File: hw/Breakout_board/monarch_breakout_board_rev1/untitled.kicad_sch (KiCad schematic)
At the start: 10 parts, among them J1 5037630491, J2 5037630291, J3 5037630291, J4 5037630291, J5 5037630291, J6 5037630291

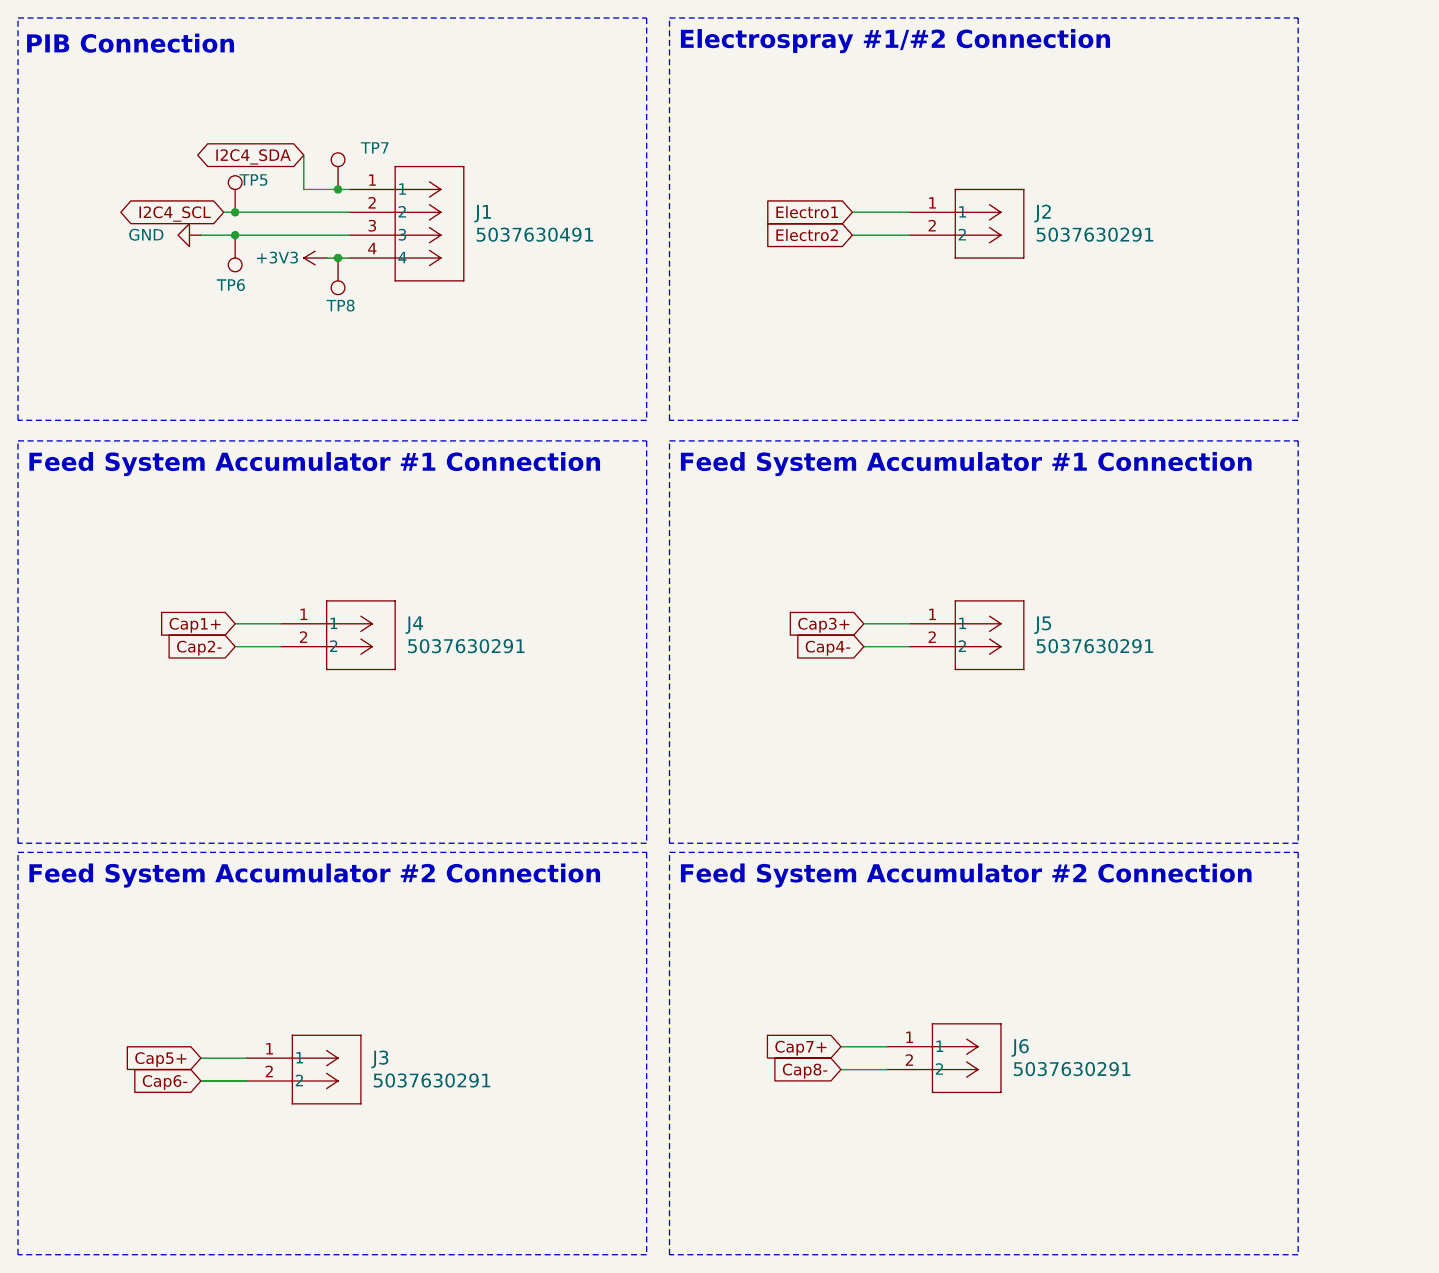
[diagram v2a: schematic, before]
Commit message: Final Breakout Board Work
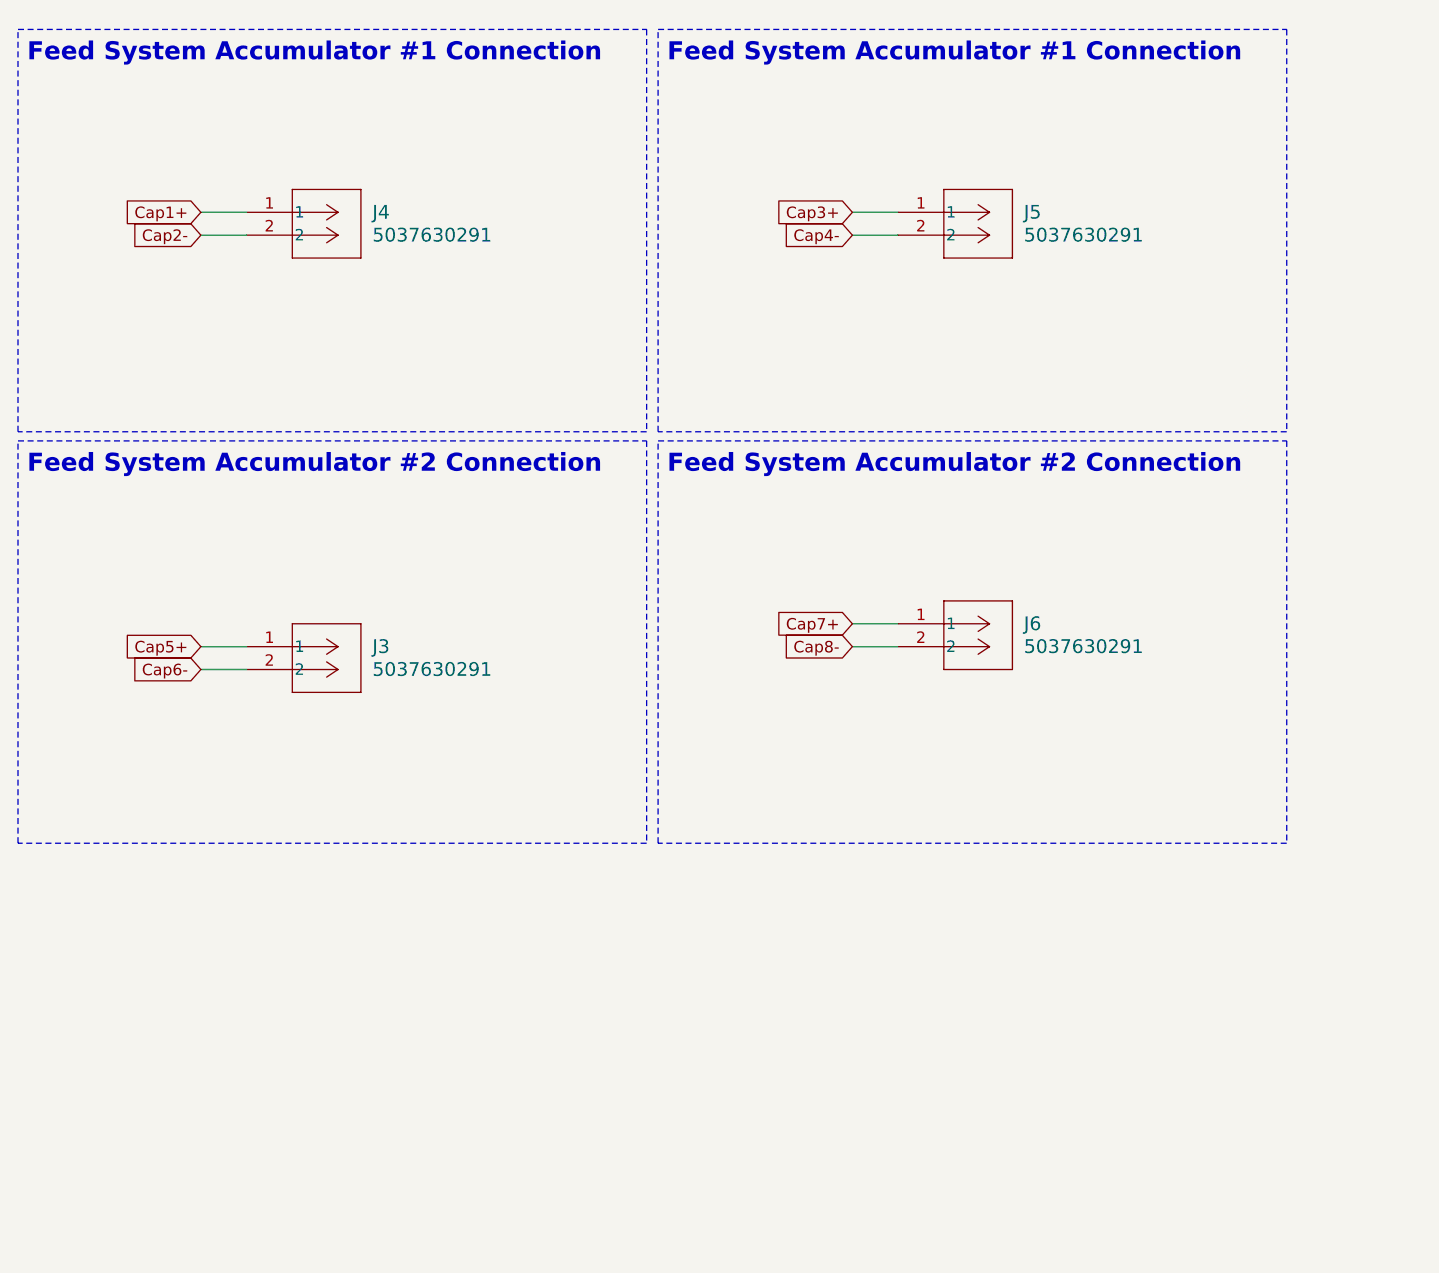
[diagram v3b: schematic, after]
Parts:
- removed J1: 5037630491, Connector 4 Pin:CONN_5037630000-SD_04_MOL, symbol 5037630491:5037630491
- removed J2: 5037630291, Connector 2 Pin:CONN_5037630000-SD_02_MOL, symbol Connectors 2 Pin:5037630291
- removed TP5, TP6, TP7, TP8: TestPoint, TestPoint:TestPoint_2Pads_Pitch2.54mm_Drill0.8mm, symbol Connector:TestPoint
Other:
- note removed: "Electrospray #1/#2 Connection"
- note removed: "PIB Connection"
- moved on the sheet: J3, J4, J5, J6

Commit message: FIXES after Review
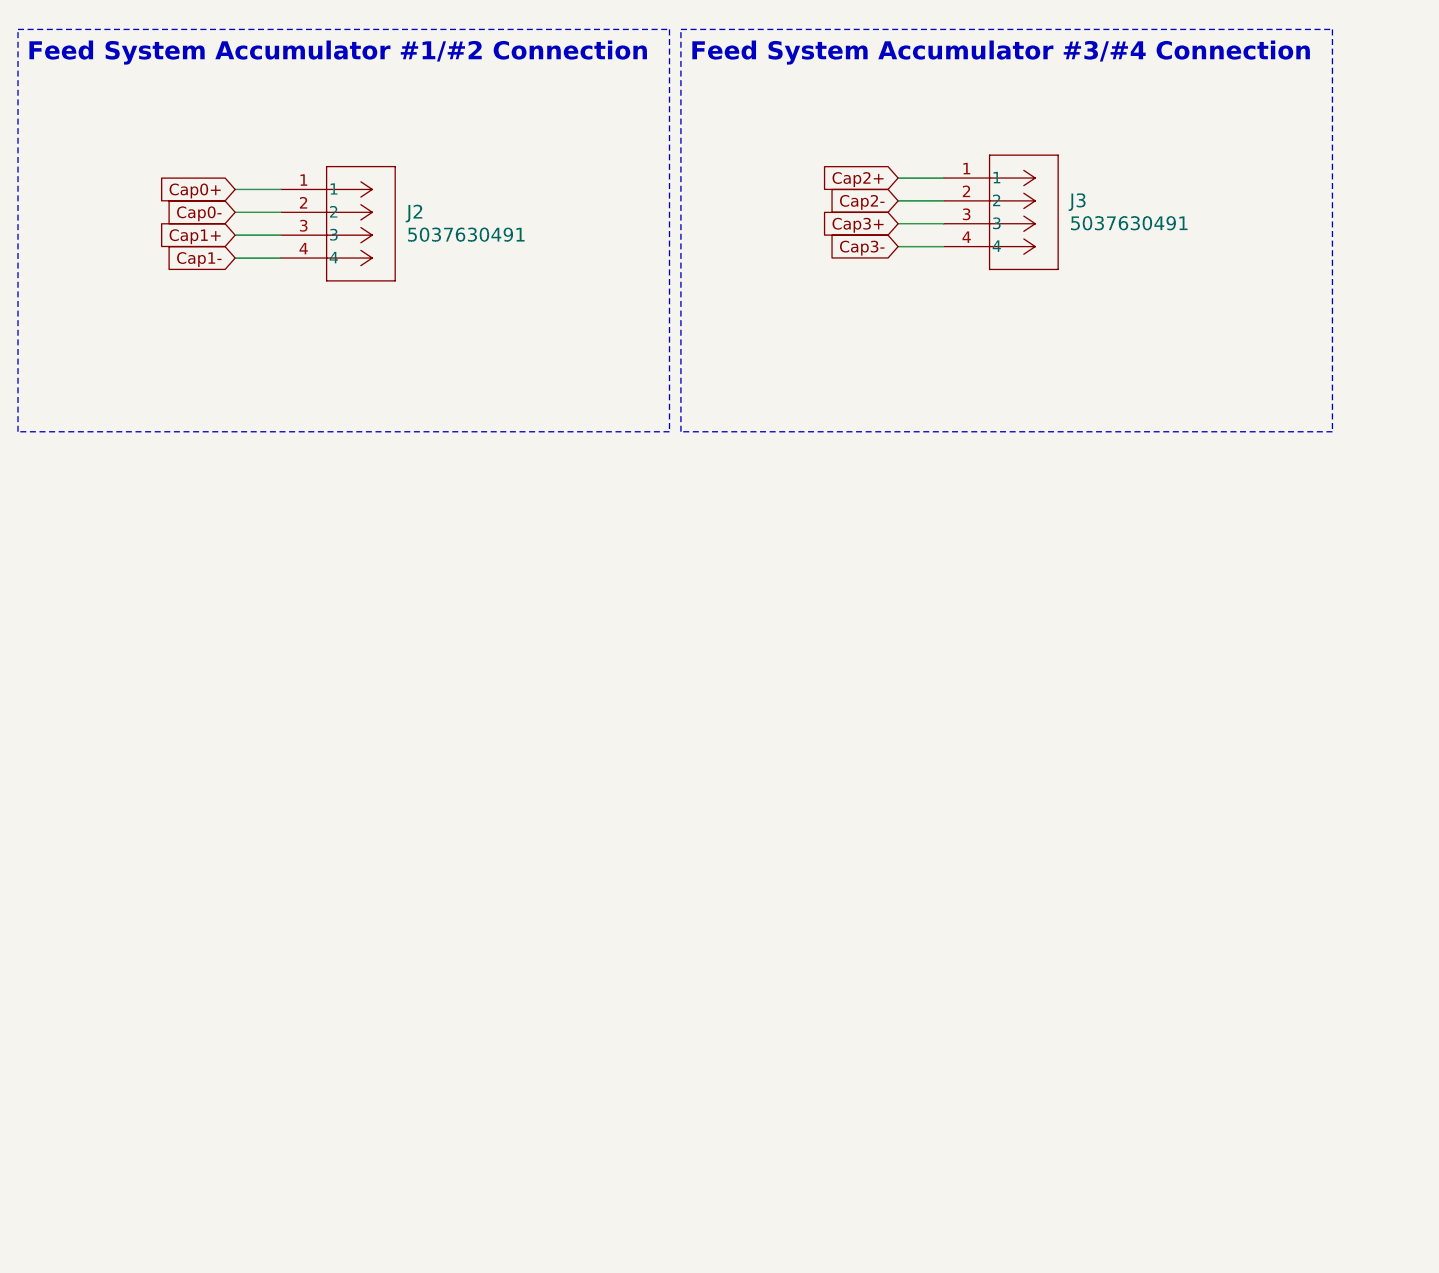
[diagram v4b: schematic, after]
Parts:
- removed J3, J4, J5, J6: 5037630291, Connector 2 Pin:CONN_5037630000-SD_02_MOL, symbol Connectors 2 Pin:5037630291
- added J2, J3: 5037630491, Connector 4 Pin:CONN_5037630000-SD_04_MOL, symbol Connectors 4 Pin:5037630491
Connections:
- net Cap1+: now also J2.3
- net Cap2-: now also J3.2
- net Cap3+: now also J3.3
- new net Cap0+: J2.1
- new net Cap0-: J2.2
- new net Cap1-: J2.4
- new net Cap2+: J3.1
- new net Cap3-: J3.4
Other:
- note added: "Feed System Accumulator #1/#2 Connection"
- note added: "Feed System Accumulator #3/#4 Connection"
- note removed: "Feed System Accumulator #1 Connection"
- note removed: "Feed System Accumulator #2 Connection"
